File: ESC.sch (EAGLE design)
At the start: 46 parts, among them U1 AMS1117-3.3

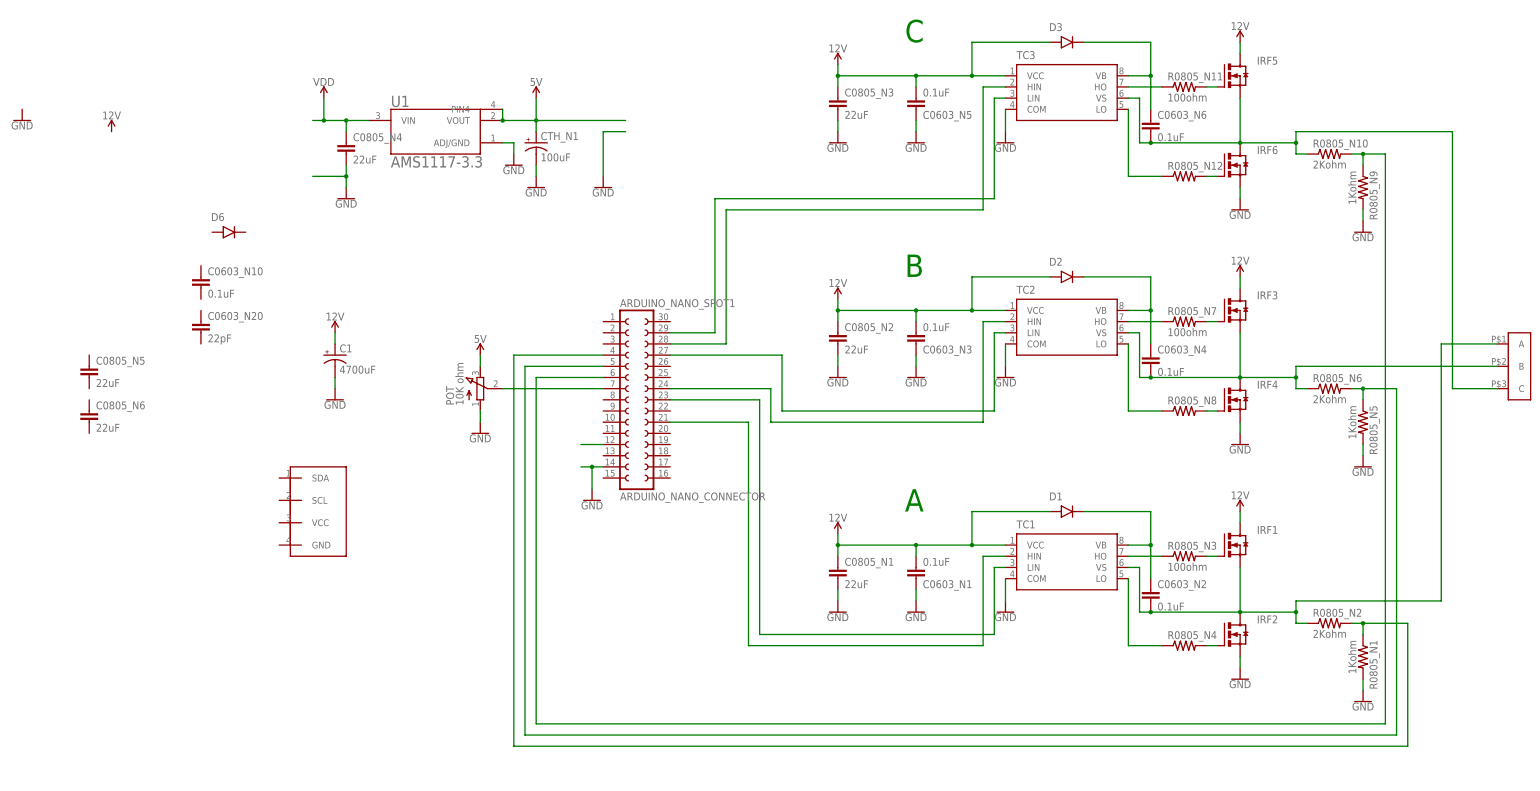
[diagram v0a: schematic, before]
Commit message: lastest edits
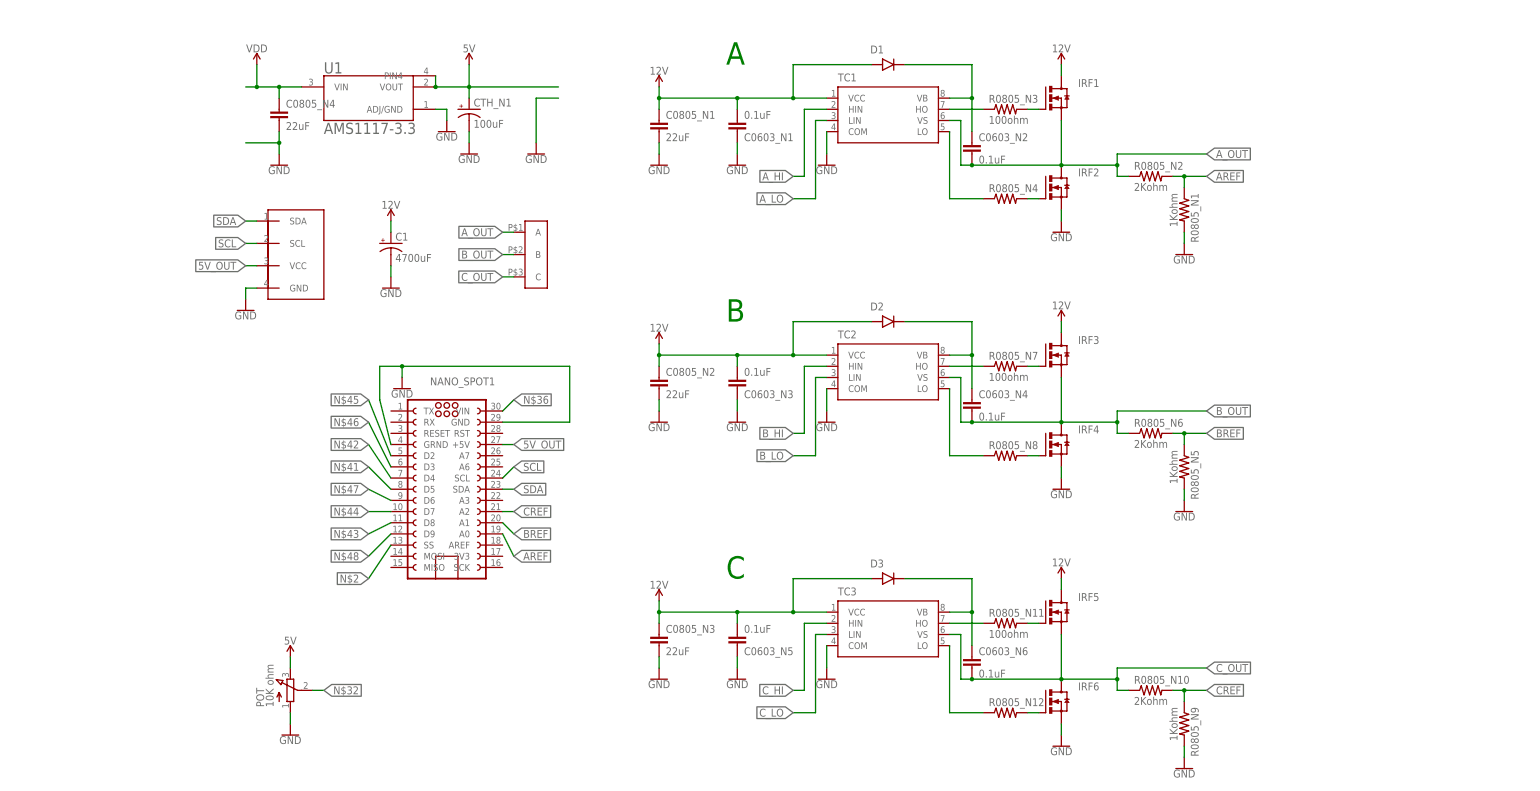
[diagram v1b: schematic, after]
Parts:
- removed ARDUINO_NANO_SPOT1: ARDUINO_NANO_CONNECTOR, TRANS_IRF3205SPBF:ARDUINO_NANO_CONNECTOR
- removed C0603_N10: 0.1uF, SparkFun-Capacitors:0.1UF-0603-25V-5%
- removed C0603_N20: 22pF, SparkFun-Capacitors:22PF-0603-50V-5%
- removed C0805_N5, C0805_N6: 22uF, SparkFun-Capacitors:22UF-0805-6.3V-20%
- removed D6: 1N4001, 1N4001:1N4001
- added NANO_SPOT1: (no value), TRANS_IRF3205SPBF:ARDUINO_NANO_CONNECTOR
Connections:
- net N$10 renamed A_OUT
- net N$13 renamed B_OUT
- net N$23 renamed C_OUT
- removed net N$16: ARDUINO_NANO_SPOT1.12
- removed net N$20: ARDUINO_NANO_SPOT1.24, TC2.HIN
- removed net N$25: ARDUINO_NANO_SPOT1.28, TC3.HIN
- removed net N$26: ARDUINO_NANO_SPOT1.29, TC3.LIN
- removed net N$30: ARDUINO_NANO_SPOT1.6, R0805_N10.2, R0805_N9.1
- removed net N$31: ARDUINO_NANO_SPOT1.7, POT.S
- removed net N$5: ARDUINO_NANO_SPOT1.21, TC1.HIN
- removed net N$7: ARDUINO_NANO_SPOT1.4, R0805_N1.1, R0805_N2.2
- removed net N$8: ARDUINO_NANO_SPOT1.23, TC1.LIN
- removed net N$9: ARDUINO_NANO_SPOT1.27, TC2.LIN
- new net 5V_OUT: NANO_SPOT1.+5V, OLED1.VCC
- new net AREF: NANO_SPOT1.A0, R0805_N1.1, R0805_N2.2
- new net A_HI: TC1.HIN
- new net A_LO: TC1.LIN
- new net BREF: NANO_SPOT1.A1, R0805_N5.1, R0805_N6.2
- new net B_HI: TC2.HIN
- new net B_LO: TC2.LIN
- new net CREF: NANO_SPOT1.A2, R0805_N10.2, R0805_N9.1
- new net C_HI: TC3.HIN
- new net C_LO: TC3.LIN
- new net N$32: POT.S
- new net N$36: NANO_SPOT1.VIN
- new net N$41: NANO_SPOT1.D5
- new net N$42: NANO_SPOT1.D4
- new net N$43: NANO_SPOT1.D8
- new net N$44: NANO_SPOT1.D7
- new net N$45: NANO_SPOT1.D2
- new net N$46: NANO_SPOT1.D3
- new net N$47: NANO_SPOT1.D6
- new net N$48: NANO_SPOT1.D9
- new net SCL: NANO_SPOT1.SCL, OLED1.SCL
- new net SDA: NANO_SPOT1.SDA, OLED1.SDA
- net GND: now also NANO_SPOT1.GND, NANO_SPOT1.GRND, OLED1.GND; no longer ARDUINO_NANO_SPOT1.14
- net N$2: now also NANO_SPOT1.SS; no longer ARDUINO_NANO_SPOT1.5, R0805_N5.1, R0805_N6.2
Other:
- moved on the sheet: C0603_N1, C0603_N2, C0603_N3, C0603_N4, C0603_N5, C0603_N6, C0805_N1, C0805_N2, C0805_N3, C0805_N4, C1, CTH_N1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
